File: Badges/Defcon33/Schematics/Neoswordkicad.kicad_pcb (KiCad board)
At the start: 2 copper layers, 217 x 77.1 mm, 81 parts, among them J1 AA Batteries, J10 Prog, J11 USB_C_Plug_USB2.0, J12 AA Conn, J2 Conn_02x03_Odd_Even, J3 Speaker, J4 Conn_02x03_Odd_Even, J5 Conn_01x08, J6 Conn_01x04, J7 Conn_02x03_Odd_Even, J8 Conn_01x04, J9 Conn_01x03, Q1 PMOS, Q2 PMOS, SW3 Lights, SW4 Sound, SW5 SW_SPDT, U1 ESP32-S3-WROOM-1, U2 MAX98357A, U3 AW20072QNR, U4 LIS2HH12, U6 TPS562243

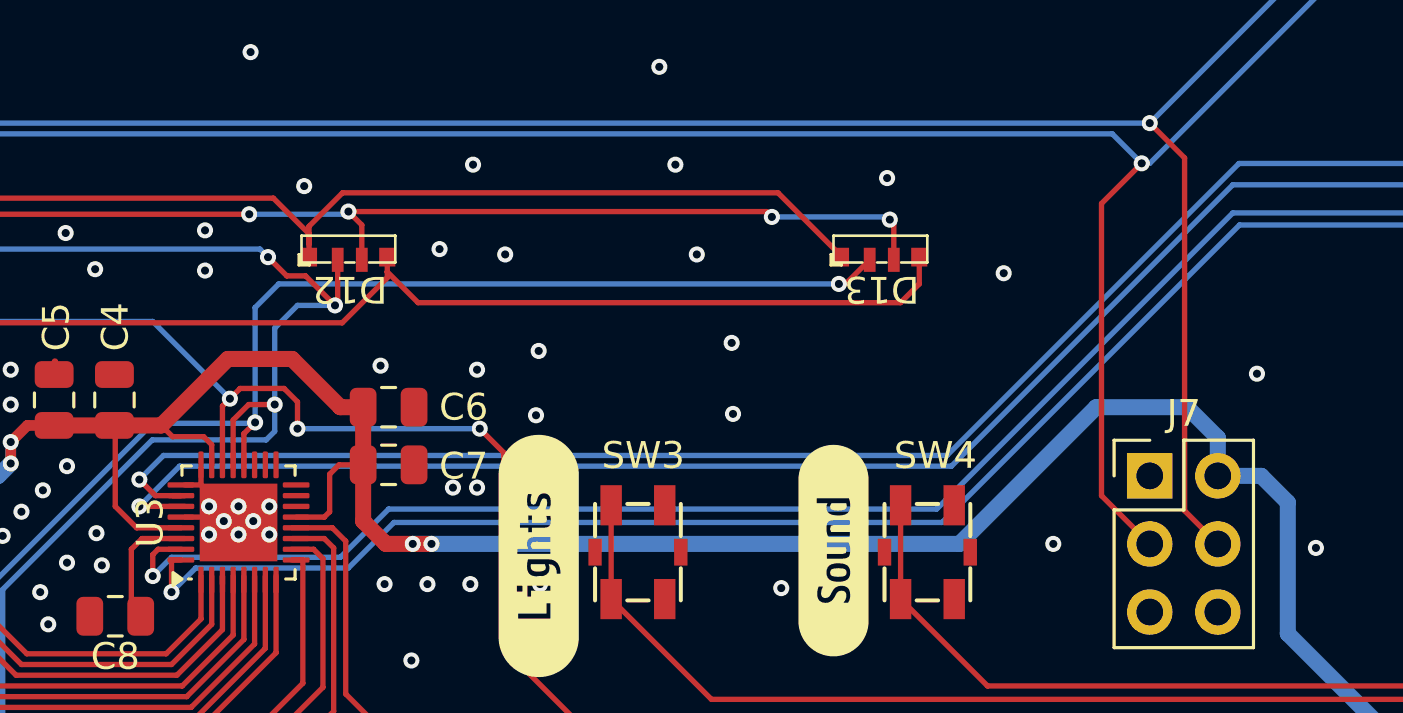
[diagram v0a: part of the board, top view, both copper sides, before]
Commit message: perhaps?
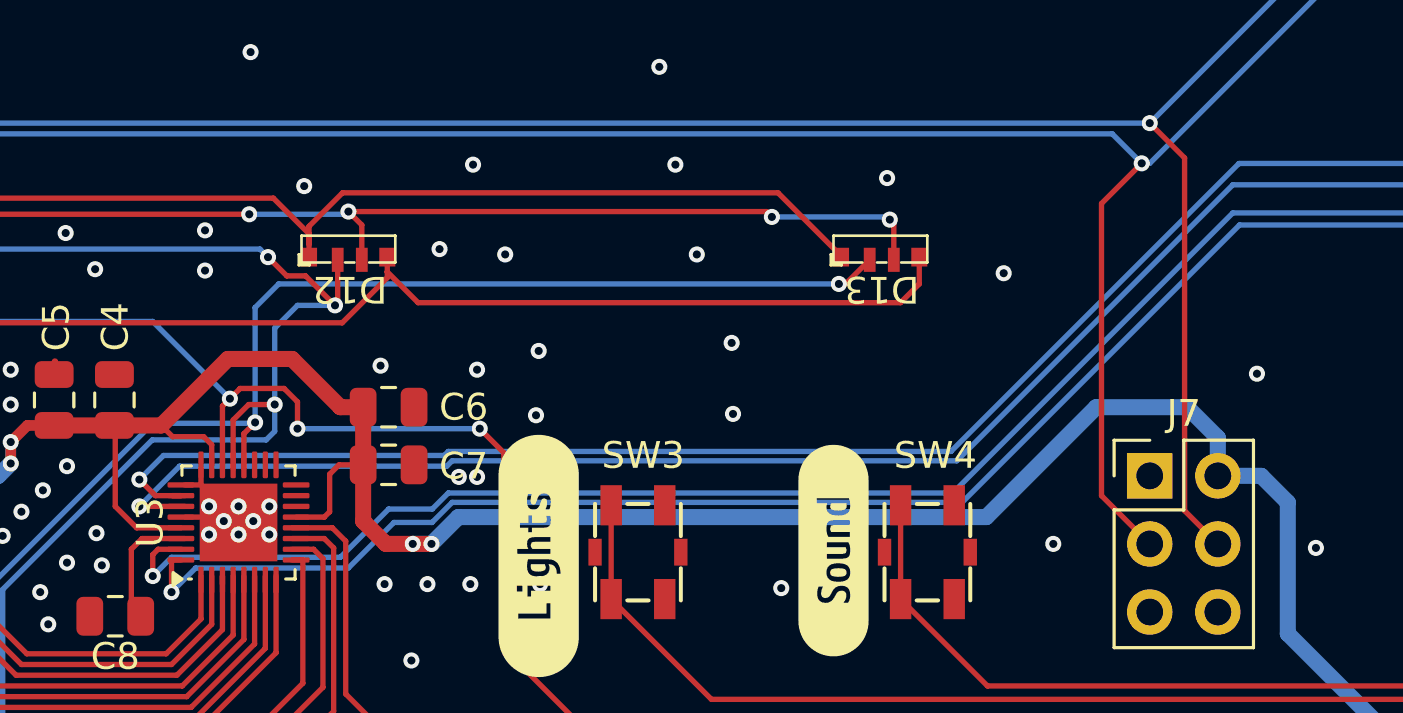
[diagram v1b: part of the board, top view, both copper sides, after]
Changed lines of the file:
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@@
 	)
 	(via
-		(at 139.6 103.6)
+		(at 139.819465 103.2)
 		(size 0.6)
 		(drill 0.3)
@@
 	)
 	(via
-		(at 140.5 103.6)
+		(at 140.5 103.2)
 		(size 0.6)
 		(drill 0.3)
@@
 	)
 	(segment
+		(start 139.570936 102.6)
+		(end 158.4 102.6)
+		(width 0.2)
+		(layer "B.Cu")
+		(net 6)
+	)
+	(segment
 		(start 202.625 90.25)
 		(end 199.8 87.425)
@@
 	)
 	(segment
-		(start 127.9 104.3)
-		(end 129.4 102.8)
+		(start 158.4 102.6)
+		(end 168.7 92.3)
 		(width 0.2)
 		(layer "B.Cu")
@@
 	)
 	(segment
-		(start 129.4 102.8)
-		(end 158.2 102.8)
+		(start 127.9 104.3)
+		(end 129.4 102.8)
 		(width 0.2)
 		(layer "B.Cu")
@@
 	)
 	(segment
-		(start 194.15 91)
-		(end 194.4 90.75)
+		(start 139.370936 102.8)
+		(end 139.570936 102.6)
 		(width 0.2)
 		(layer "B.Cu")
@@
 	)
 	(segment
-		(start 168.7 92.3)
-		(end 176.65 92.3)
+		(start 129.4 102.8)
+		(end 139.370936 102.8)
 		(width 0.2)
 		(layer "B.Cu")
@@
 	)
 	(segment
-		(start 158.2 102.8)
-		(end 168.7 92.3)
+		(start 194.15 91)
+		(end 194.4 90.75)
+		(width 0.2)
+		(layer "B.Cu")
+		(net 6)
+	)
+	(segment
+		(start 168.7 92.3)
+		(end 176.65 92.3)
 		(width 0.2)
 		(layer "B.Cu")
@@
 	)
 	(segment
-		(start 158.034314 102.4)
-		(end 168.928553 91.505761)
+		(start 128.8 102.4)
+		(end 139.275961 102.4)
 		(width 0.2)
 		(layer "B.Cu")
@@
 	)
 	(segment
-		(start 168.928553 91.505761)
-		(end 176.755761 91.505761)
+		(start 127.9 103.3)
+		(end 128.8 102.4)
 		(width 0.2)
 		(layer "B.Cu")
@@
 	)
 	(segment
-		(start 128.8 102.4)
-		(end 158.034314 102.4)
+		(start 139.425962 102.25)
+		(end 158.184314 102.25)
+		(width 0.2)
+		(layer "B.Cu")
+		(net 7)
+	)
+	(segment
+		(start 139.275961 102.4)
+		(end 139.425962 102.25)
 		(width 0.2)
 		(layer "B.Cu")
@@
 	)
 	(segment
-		(start 127.9 103.3)
-		(end 128.8 102.4)
+		(start 168.928553 91.505761)
+		(end 176.755761 91.505761)
 		(width 0.2)
 		(layer "B.Cu")
@@
 	)
 	(segment
+		(start 158.184314 102.25)
+		(end 168.928553 91.505761)
+		(width 0.2)
+		(layer "B.Cu")
+		(net 7)
+	)
+	(segment
 		(start 240.274933 95.65)
 		(end 242.6 95.65)
@@
 	)
 	(segment
-		(start 157.85 104.9)
-		(end 168.95 93.8)
-		(width 0.2)
-		(layer "B.Cu")
-		(net 73)
-	)
-	(segment
-		(start 130 106.6)
-		(end 135.7 106.6)
+		(start 176.95 93.8)
+		(end 179.6 91.15)
 		(width 0.2)
 		(layer "B.Cu")
@@
 	)
 	(segment
-		(start 168.95 93.8)
-		(end 176.95 93.8)
+		(start 158.6 104.15)
+		(end 168.95 93.8)
 		(width 0.2)
 		(layer "B.Cu")
@@
 	)
 	(segment
-		(start 129.1 107.5)
-		(end 130 106.6)
+		(start 130 106.6)
+		(end 135.7 106.6)
 		(width 0.2)
 		(layer "B.Cu")
@@
 	)
 	(segment
-		(start 137.4 104.9)
-		(end 157.85 104.9)
+		(start 168.95 93.8)
+		(end 176.95 93.8)
 		(width 0.2)
 		(layer "B.Cu")
@@
 	)
 	(segment
+		(start 129.1 107.5)
+		(end 130 106.6)
+		(width 0.2)
+		(layer "B.Cu")
+		(net 73)
+	)
+	(segment
 		(start 195.65 80.95)
 		(end 194.85 80.15)
@@
 	)
 	(segment
-		(start 135.7 106.6)
-		(end 137.4 104.9)
+		(start 138.822182 104.9)
+		(end 139.572183 104.15)
 		(width 0.2)
 		(layer "B.Cu")
@@
 	)
 	(segment
-		(start 176.95 93.8)
-		(end 179.6 91.15)
+		(start 135.7 106.6)
+		(end 137.4 104.9)
 		(width 0.2)
 		(layer "B.Cu")
@@
 	)
 	(segment
+		(start 139.572183 104.15)
+		(end 158.6 104.15)
+		(width 0.2)
+		(layer "B.Cu")
+		(net 73)
+	)
+	(segment
+		(start 137.4 104.9)
+		(end 138.822182 104.9)
+		(width 0.2)
+		(layer "B.Cu")
+		(net 73)
+	)
+	(segment
 		(start 128.4 106.9)
 		(end 128.4 106.1)
@@
 	)
 	(segment
+		(start 128.4 106.9)
+		(end 129.1 106.2)
+		(width 0.2)
+		(layer "B.Cu")
+		(net 74)
+	)
+	(segment
 		(start 193.15 87.5)
 		(end 195 85.65)
@@
 	)
 	(segment
-		(start 195 82.8)
-		(end 195 81.95)
+		(start 135.4 106.2)
+		(end 137.2 104.4)
 		(width 0.2)
 		(layer "B.Cu")
@@
 	)
 	(segment
-		(start 157.65 104.4)
-		(end 168.7 93.35)
+		(start 137.2 104.4)
+		(end 138.827207 104.4)
 		(width 0.2)
 		(layer "B.Cu")
@@
 	)
 	(segment
-		(start 135.4 106.2)
-		(end 137.2 104.4)
+		(start 195 82.8)
+		(end 195 81.95)
 		(width 0.2)
 		(layer "B.Cu")
@@
 	)
 	(segment
-		(start 168.7 93.35)
-		(end 176.75 93.35)
+		(start 179.681206 90.418794)
+		(end 179.681206 90.343617)
 		(width 0.2)
 		(layer "B.Cu")
@@
 	)
 	(segment
-		(start 179.681206 90.418794)
-		(end 179.681206 90.343617)
+		(start 129.1 106.2)
+		(end 135.4 106.2)
 		(width 0.2)
 		(layer "B.Cu")
@@
 	)
 	(segment
-		(start 128.4 106.9)
-		(end 129.1 106.2)
+		(start 138.827207 104.4)
+		(end 139.427208 103.8)
 		(width 0.2)
 		(layer "B.Cu")
@@
 	)
 	(segment
-		(start 129.1 106.2)
-		(end 135.4 106.2)
+		(start 139.427208 103.8)
+		(end 158.25 103.8)
 		(width 0.2)
 		(layer "B.Cu")
@@
 	)
 	(segment
-		(start 137.2 104.4)
-		(end 157.65 104.4)
+		(start 168.7 93.35)
+		(end 176.75 93.35)
+		(width 0.2)
+		(layer "B.Cu")
+		(net 74)
+	)
+	(segment
+		(start 158.25 103.8)
+		(end 168.7 93.35)
 		(width 0.2)
 		(layer "B.Cu")
@@
 	)
 	(segment
-		(start 167 100.6)
-		(end 168.14 101.74)
-		(width 0.6)
-		(layer "B.Cu")
-		(net 81)
-	)
-	(segment
 		(start 195 70.1)
 		(end 196.2 71.3)
@@
 	)
 	(segment
-		(start 138.8 105.7)
-		(end 158.5 105.7)
-		(width 0.6)
-		(layer "B.Cu")
-		(net 81)
-	)
-	(segment
 		(start 195 70.1)
 		(end 214.7 70.1)
@@
 	)
 	(segment
-		(start 158.5 105.7)
-		(end 163.6 100.6)
-		(width 0.6)
-		(layer "B.Cu")
-		(net 81)
-	)
-	(segment
 		(start 123.1 101.9)
 		(end 123.1 102.7)
@@
 	)
 	(segment
+		(start 138.8 105.7)
+		(end 139.8 104.7)
+		(width 0.6)
+		(layer "B.Cu")
+		(net 81)
+	)
+	(segment
 		(start 204.5 95.2)
 		(end 205.5 94.2)
@@
 	)
 	(segment
-		(start 163.6 100.6)
-		(end 167 100.6)
-		(width 0.6)
-		(layer "B.Cu")
-		(net 81)
-	)
-	(segment
 		(start 169.761482 103.161482)
 		(end 168.14 103.161482)
@@
 	)
 	(segment
-		(start 168.14 101.74)
-		(end 168.14 103.161482)
+		(start 159.5 104.7)
+		(end 163.6 100.6)
+		(width 0.6)
+		(layer "B.Cu")
+		(net 81)
+	)
+	(segment
+		(start 163.6 100.6)
+		(end 167 100.6)
 		(width 0.6)
 		(layer "B.Cu")
@@
 	)
 	(segment
+		(start 139.8 104.7)
+		(end 159.5 104.7)
+		(width 0.6)
+		(layer "B.Cu")
+		(net 81)
+	)
+	(segment
 		(start 225.1 92.7)
 		(end 225.1 102.4)
@@
 	)
 	(segment
+		(start 168.14 101.74)
+		(end 168.14 103.161482)
+		(width 0.6)
+		(layer "B.Cu")
+		(net 81)
+	)
+	(segment
 		(start 98.8 98.7)
 		(end 116.199999 98.7)
@@
 		(width 0.6)
 		(layer "B.Cu")
+		(net 81)
+	)
+	(segment
+		(start 167 100.6)
+		(end 168.14 101.74)
+		(width 0.6)
+		(layer "B.Cu")
